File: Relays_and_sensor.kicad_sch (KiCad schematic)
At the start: 24 parts, among them J4 Screw_Terminal_01x02, J5 Screw_Terminal_01x02, J6 Screw_Terminal_01x02, J7 Screw_Terminal_01x02, J8 Screw_Terminal_01x02, K1 1461103-1, K2 1461103-1, K3 1461103-1, K4 1461103-1, Q1 ZTX450, Q2 ZTX450, Q3 ZTX450, Q4 ZTX450

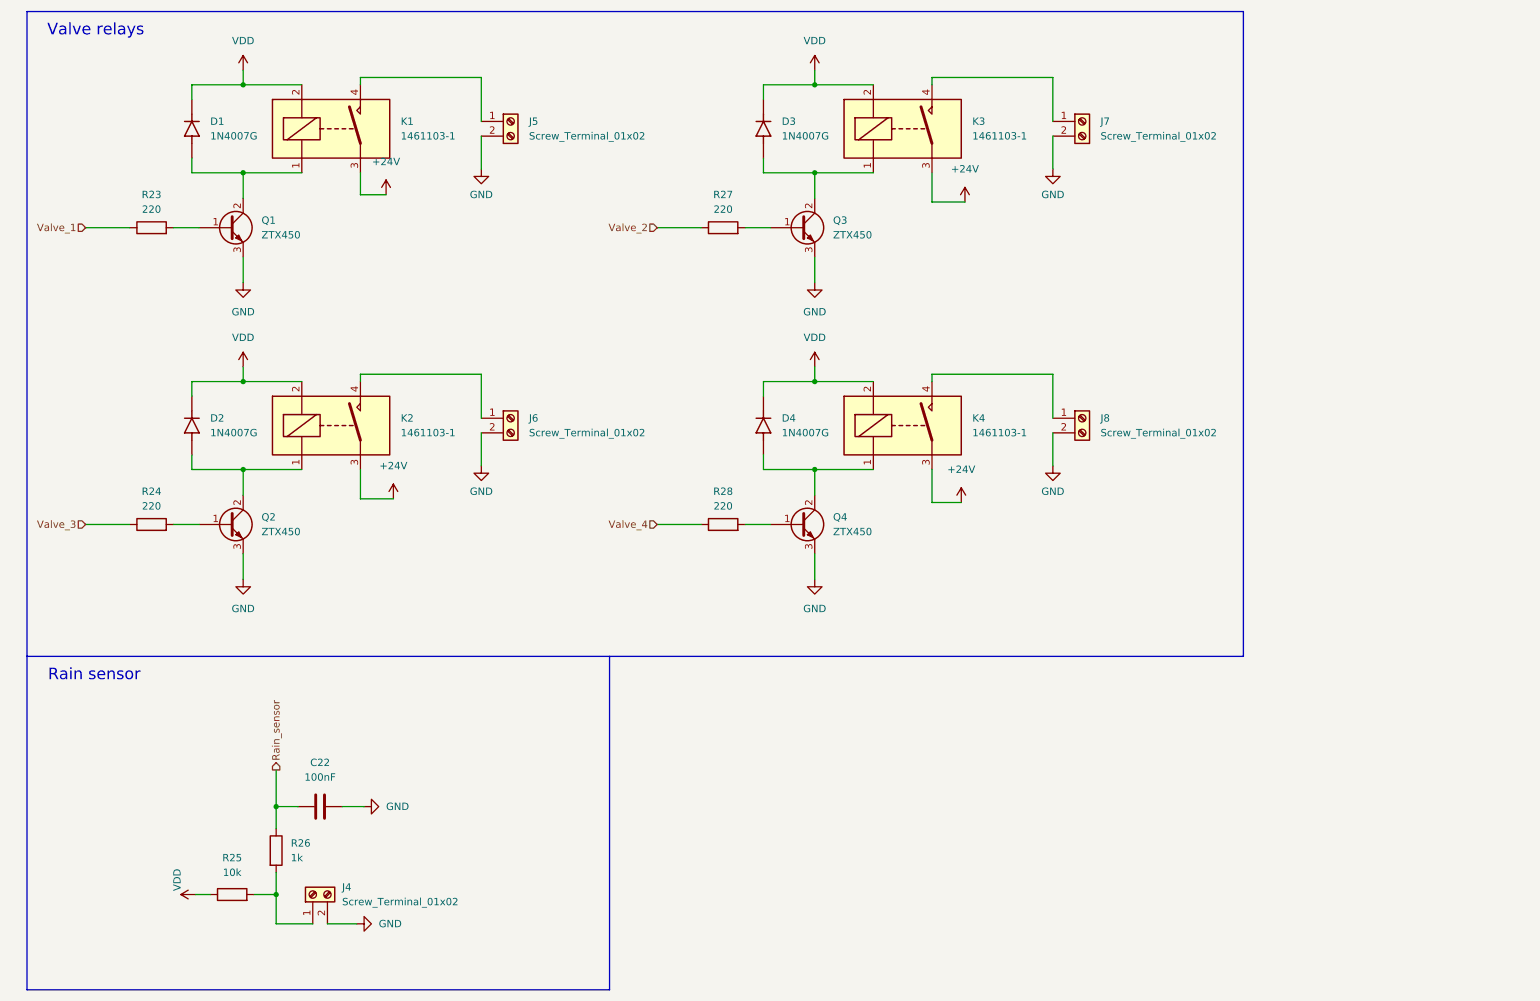
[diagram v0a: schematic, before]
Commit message: Isolation
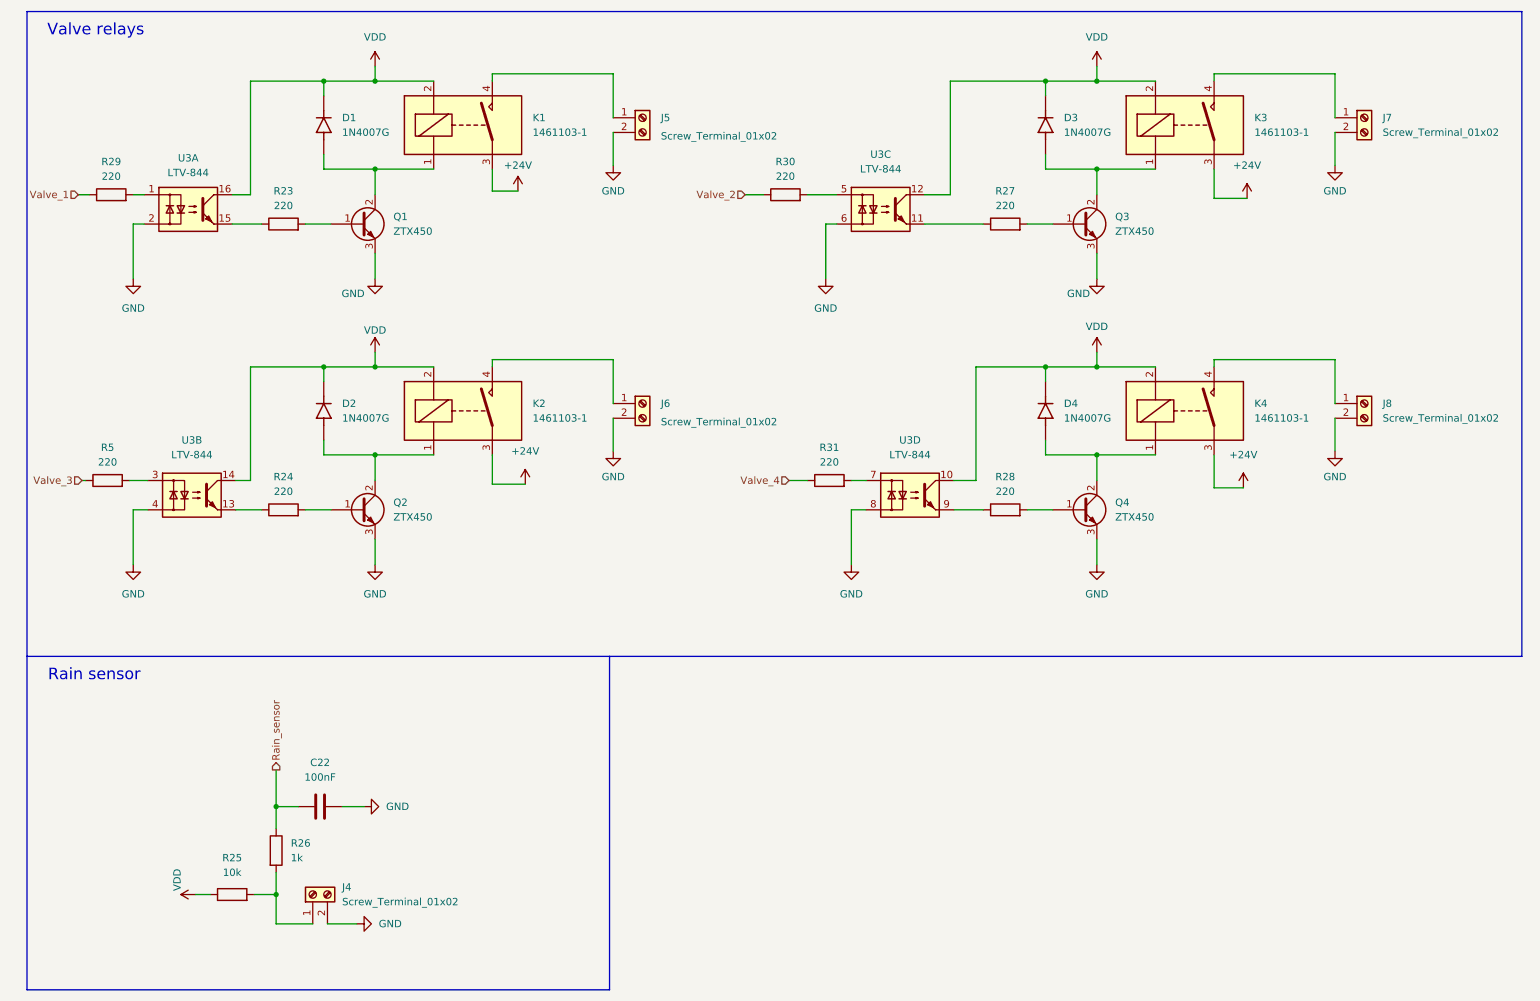
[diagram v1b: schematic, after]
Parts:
- added R29, R30, R31, R5: 220, symbol Device:R
- added U3: LTV-844, Package_DIP:DIP-16_W7.62mm, symbol Isolator:LTV-844
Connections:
- net GND: now also U3.2, U3.4, U3.6, U3.8
- net VDD: now also U3.10, U3.12, U3.14, U3.16
- net Valve_1: now also R29.1; no longer R23.1
- net Valve_2: now also R30.1; no longer R27.1
- net Valve_3: now also R5.1; no longer R24.1
- net Valve_4: now also R31.1; no longer R28.1
- new net: R29.2, U3.1
- new net: R24.1, U3.13
- new net: R5.2, U3.3
- new net: R31.2, U3.7
- new net: R30.2, U3.5
- new net: R28.1, U3.9
- new net: R27.1, U3.11
- new net: R23.1, U3.15
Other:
- moved on the sheet: D1, D2, D3, D4, J5, J6, J7, J8, K1, K2, K3, K4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

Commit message: Rezystory, kondensatory, cewka - footprints
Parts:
- C22: footprint (none) -> Capacitor_SMD:C_0603_1608Metric
- D1, D2, D3, D4: footprint DIOAD1036W78L470D235 -> (none)
- R23, R24, R25, R26, R27, R28, R29, R30, R31, R5: footprint (none) -> Resistor_SMD:R_0603_1608Metric
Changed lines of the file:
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@@
       (effects (font (size 1.27 1.27)) (justify right))
     )
-    (property "Footprint" "DIOAD1036W78L470D235" (id 2) (at 66.04 36.83 0)
+    (property "Footprint" "" (id 2) (at 66.04 36.83 0)
       (effects (font (size 1.27 1.27)) (justify left bottom) hide)
     )
@@
     (property "Reference" "R25" (id 0) (at 50.165 163.83 90))
     (property "Value" "10k" (id 1) (at 50.165 166.37 90))
-    (property "Footprint" "" (id 2) (at 50.165 171.958 90)
+    (property "Footprint" "Resistor_SMD:R_0603_1608Metric" (id 2) (at 50.165 171.958 90)
       (effects (font (size 1.27 1.27)) hide)
     )
@@
     (property "Reference" "R29" (id 0) (at 29.21 43.18 90))
     (property "Value" "220" (id 1) (at 29.21 45.72 90))
-    (property "Footprint" "" (id 2) (at 29.21 50.673 90)
+    (property "Footprint" "Resistor_SMD:R_0603_1608Metric" (id 2) (at 29.21 50.673 90)
       (effects (font (size 1.27 1.27)) hide)
     )
@@
     (property "Reference" "R31" (id 0) (at 153.67 92.71 90))
     (property "Value" "220" (id 1) (at 153.67 95.25 90))
-    (property "Footprint" "" (id 2) (at 153.67 100.203 90)
+    (property "Footprint" "Resistor_SMD:R_0603_1608Metric" (id 2) (at 153.67 100.203 90)
       (effects (font (size 1.27 1.27)) hide)
     )
@@
     (property "Reference" "R5" (id 0) (at 28.575 92.71 90))
     (property "Value" "220" (id 1) (at 28.575 95.25 90))
-    (property "Footprint" "" (id 2) (at 28.575 100.203 90)
+    (property "Footprint" "Resistor_SMD:R_0603_1608Metric" (id 2) (at 28.575 100.203 90)
       (effects (font (size 1.27 1.27)) hide)
     )
@@
       (effects (font (size 1.27 1.27)) (justify right))
     )
-    (property "Footprint" "DIOAD1036W78L470D235" (id 2) (at 66.04 86.36 0)
+    (property "Footprint" "" (id 2) (at 66.04 86.36 0)
       (effects (font (size 1.27 1.27)) (justify left bottom) hide)
     )
@@
     (property "Reference" "R30" (id 0) (at 146.05 43.18 90))
     (property "Value" "220" (id 1) (at 146.05 45.72 90))
-    (property "Footprint" "" (id 2) (at 146.05 50.673 90)
+    (property "Footprint" "Resistor_SMD:R_0603_1608Metric" (id 2) (at 146.05 50.673 90)
       (effects (font (size 1.27 1.27)) hide)
     )
@@
     (property "Reference" "R24" (id 0) (at 59.055 97.79 90))
     (property "Value" "220" (id 1) (at 59.055 100.33 90))
-    (property "Footprint" "" (id 2) (at 59.055 105.283 90)
+    (property "Footprint" "Resistor_SMD:R_0603_1608Metric" (id 2) (at 59.055 105.283 90)
       (effects (font (size 1.27 1.27)) hide)
     )
@@
       (effects (font (size 1.27 1.27)) (justify right))
     )
-    (property "Footprint" "DIOAD1036W78L470D235" (id 2) (at 191.135 36.83 0)
+    (property "Footprint" "" (id 2) (at 191.135 36.83 0)
       (effects (font (size 1.27 1.27)) (justify left bottom) hide)
     )
@@
     (property "Reference" "R28" (id 0) (at 184.15 97.79 90))
     (property "Value" "220" (id 1) (at 184.15 100.33 90))
-    (property "Footprint" "" (id 2) (at 184.15 105.283 90)
+    (property "Footprint" "Resistor_SMD:R_0603_1608Metric" (id 2) (at 184.15 105.283 90)
       (effects (font (size 1.27 1.27)) hide)
     )
@@
       (effects (font (size 1.27 1.27)) (justify right))
     )
-    (property "Footprint" "DIOAD1036W78L470D235" (id 2) (at 191.135 86.36 0)
+    (property "Footprint" "" (id 2) (at 191.135 86.36 0)
       (effects (font (size 1.27 1.27)) (justify left bottom) hide)
     )
@@
     (property "Reference" "C22" (id 0) (at 65.405 147.32 90))
     (property "Value" "100nF" (id 1) (at 65.405 149.86 90))
-    (property "Footprint" "" (id 2) (at 69.215 153.9748 0)
+    (property "Footprint" "Capacitor_SMD:C_0603_1608Metric" (id 2) (at 69.215 153.9748 0)
       (effects (font (size 1.27 1.27)) hide)
     )
@@
       (effects (font (size 1.27 1.27)) (justify left))
     )
-    (property "Footprint" "" (id 2) (at 56.007 162.56 90)
+    (property "Footprint" "Resistor_SMD:R_0603_1608Metric" (id 2) (at 56.007 162.56 90)
       (effects (font (size 1.27 1.27)) hide)
     )
@@
     (property "Reference" "R27" (id 0) (at 184.15 48.26 90))
     (property "Value" "220" (id 1) (at 184.15 50.8 90))
-    (property "Footprint" "" (id 2) (at 184.15 55.753 90)
+    (property "Footprint" "Resistor_SMD:R_0603_1608Metric" (id 2) (at 184.15 55.753 90)
       (effects (font (size 1.27 1.27)) hide)
     )
@@
     (property "Reference" "R23" (id 0) (at 59.055 48.26 90))
     (property "Value" "220" (id 1) (at 59.055 50.8 90))
-    (property "Footprint" "" (id 2) (at 59.055 55.753 90)
-      (effects (font (size 1.27 1.27)) hide)
-    )
+    (property "Footprint" "Resistor_SMD:R_0603_1608Metric" (id 2) (at 59.055 55.753 90)
+      (effects (font (size 1.27 1.27)) hide)
+    )

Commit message: footprints
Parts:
- D1, D2, D3, D4: footprint (none) -> 1N4007G:DIOAD1036W78L470D235
- J4, J5, J6, J7, J8: footprint (none) -> TerminalBlock:TerminalBlock_bornier-2_P5.08mm
- K1, K2, K3, K4: footprint (none) -> Project_lic_footprints_AM:OJ_OJE
- Q1, Q2, Q3, Q4: footprint (none) -> eec:TO92250P510H770-3
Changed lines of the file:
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@@
       (effects (font (size 1.27 1.27)) (justify right))
     )
-    (property "Footprint" "" (id 2) (at 66.04 36.83 0)
+    (property "Footprint" "1N4007G:DIOAD1036W78L470D235" (id 2) (at 66.04 36.83 0)
       (effects (font (size 1.27 1.27)) (justify left bottom) hide)
     )
@@
       (effects (font (size 1.27 1.27)) (justify left))
     )
-    (property "Footprint" "" (id 2) (at 77.47 51.435 0)
+    (property "Footprint" "eec:TO92250P510H770-3" (id 2) (at 77.47 51.435 0)
       (effects (font (size 1.27 1.27)) hide)
     )
@@
       (effects (font (size 1.27 1.27)) (justify left))
     )
-    (property "Footprint" "" (id 2) (at 205.105 91.44 0)
+    (property "Footprint" "Project_lic_footprints_AM:OJ_OJE" (id 2) (at 205.105 91.44 0)
       (effects (font (size 1.27 1.27)) hide)
     )
@@
       (effects (font (size 1.27 1.27)) (justify left))
     )
-    (property "Footprint" "" (id 2) (at 246.38 35.56 0)
+    (property "Footprint" "TerminalBlock:TerminalBlock_bornier-2_P5.08mm" (id 2) (at 246.38 35.56 0)
       (effects (font (size 1.27 1.27)) hide)
     )
@@
       (effects (font (size 1.27 1.27)) (justify left))
     )
-    (property "Footprint" "" (id 2) (at 121.285 35.56 0)
+    (property "Footprint" "TerminalBlock:TerminalBlock_bornier-2_P5.08mm" (id 2) (at 121.285 35.56 0)
       (effects (font (size 1.27 1.27)) hide)
     )
@@
       (effects (font (size 1.27 1.27)) (justify right))
     )
-    (property "Footprint" "" (id 2) (at 66.04 86.36 0)
+    (property "Footprint" "1N4007G:DIOAD1036W78L470D235" (id 2) (at 66.04 86.36 0)
       (effects (font (size 1.27 1.27)) (justify left bottom) hide)
     )
@@
       (effects (font (size 1.27 1.27)) (justify left))
     )
-    (property "Footprint" "" (id 2) (at 246.38 85.09 0)
+    (property "Footprint" "TerminalBlock:TerminalBlock_bornier-2_P5.08mm" (id 2) (at 246.38 85.09 0)
       (effects (font (size 1.27 1.27)) hide)
     )
@@
       (effects (font (size 1.27 1.27)) (justify right))
     )
-    (property "Footprint" "" (id 2) (at 191.135 36.83 0)
+    (property "Footprint" "1N4007G:DIOAD1036W78L470D235" (id 2) (at 191.135 36.83 0)
       (effects (font (size 1.27 1.27)) (justify left bottom) hide)
     )
@@
       (effects (font (size 1.27 1.27)) (justify left))
     )
-    (property "Footprint" "" (id 2) (at 202.565 100.965 0)
+    (property "Footprint" "eec:TO92250P510H770-3" (id 2) (at 202.565 100.965 0)
       (effects (font (size 1.27 1.27)) hide)
     )
@@
       (effects (font (size 1.27 1.27)) (justify right))
     )
-    (property "Footprint" "" (id 2) (at 191.135 86.36 0)
+    (property "Footprint" "1N4007G:DIOAD1036W78L470D235" (id 2) (at 191.135 86.36 0)
       (effects (font (size 1.27 1.27)) (justify left bottom) hide)
     )
@@
       (effects (font (size 1.27 1.27)) (justify left))
     )
-    (property "Footprint" "" (id 2) (at 80.01 91.44 0)
+    (property "Footprint" "Project_lic_footprints_AM:OJ_OJE" (id 2) (at 80.01 91.44 0)
       (effects (font (size 1.27 1.27)) hide)
     )
@@
       (effects (font (size 1.27 1.27)) (justify left))
     )
-    (property "Footprint" "" (id 2) (at 121.285 85.09 0)
+    (property "Footprint" "TerminalBlock:TerminalBlock_bornier-2_P5.08mm" (id 2) (at 121.285 85.09 0)
       (effects (font (size 1.27 1.27)) hide)
     )
@@
       (effects (font (size 1.27 1.27)) (justify left))
     )
-    (property "Footprint" "" (id 2) (at 77.47 100.965 0)
+    (property "Footprint" "eec:TO92250P510H770-3" (id 2) (at 77.47 100.965 0)
       (effects (font (size 1.27 1.27)) hide)
     )
@@
       (effects (font (size 1.27 1.27)) (justify left))
     )
-    (property "Footprint" "" (id 2) (at 202.565 51.435 0)
+    (property "Footprint" "eec:TO92250P510H770-3" (id 2) (at 202.565 51.435 0)
       (effects (font (size 1.27 1.27)) hide)
     )
@@
       (effects (font (size 1.27 1.27)) (justify left))
     )
-    (property "Footprint" "" (id 2) (at 205.105 41.91 0)
+    (property "Footprint" "Project_lic_footprints_AM:OJ_OJE" (id 2) (at 205.105 41.91 0)
       (effects (font (size 1.27 1.27)) hide)
     )
@@
       (effects (font (size 1.27 1.27)) (justify right))
     )
-    (property "Footprint" "" (id 2) (at 64.135 170.18 0)
+    (property "Footprint" "TerminalBlock:TerminalBlock_bornier-2_P5.08mm" (id 2) (at 64.135 170.18 0)
       (effects (font (size 1.27 1.27)) hide)
     )
@@
       (effects (font (size 1.27 1.27)) (justify left))
     )
-    (property "Footprint" "" (id 2) (at 80.01 41.91 0)
-      (effects (font (size 1.27 1.27)) hide)
-    )
+    (property "Footprint" "Project_lic_footprints_AM:OJ_OJE" (id 2) (at 80.01 41.91 0)
+      (effects (font (size 1.27 1.27)) hide)
+    )
